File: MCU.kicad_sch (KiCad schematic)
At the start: 17 parts, among them J1 Conn_01x05_Socket, SW1 SW_Push, U1 STM32F405RGT6, Y1 8MHz 10ppm

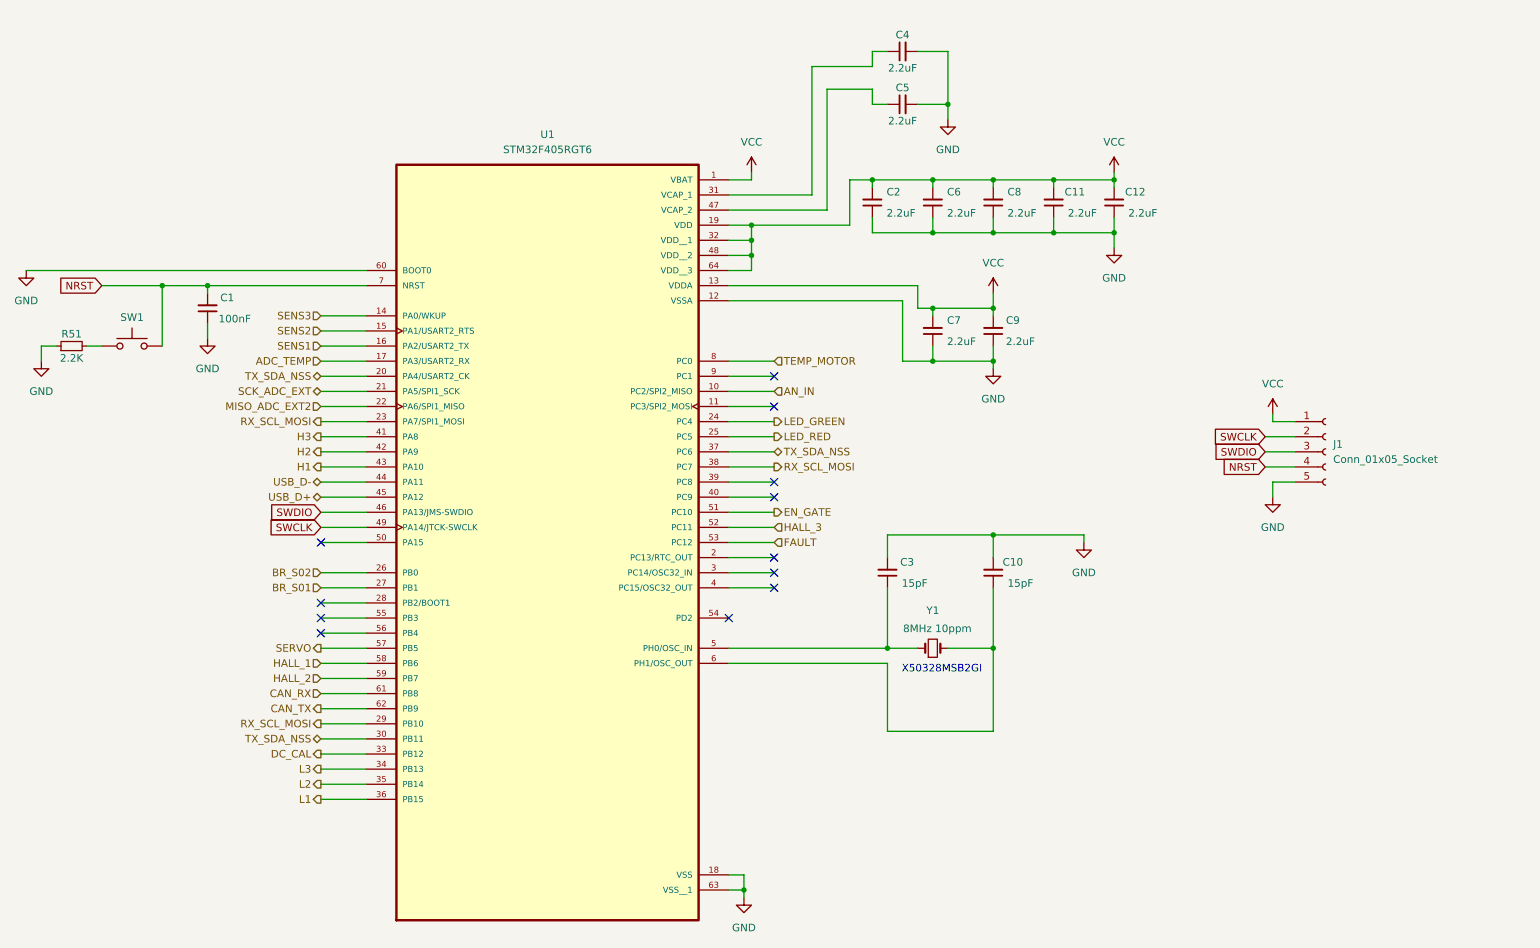
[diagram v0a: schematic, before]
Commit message: finishing+microchecking
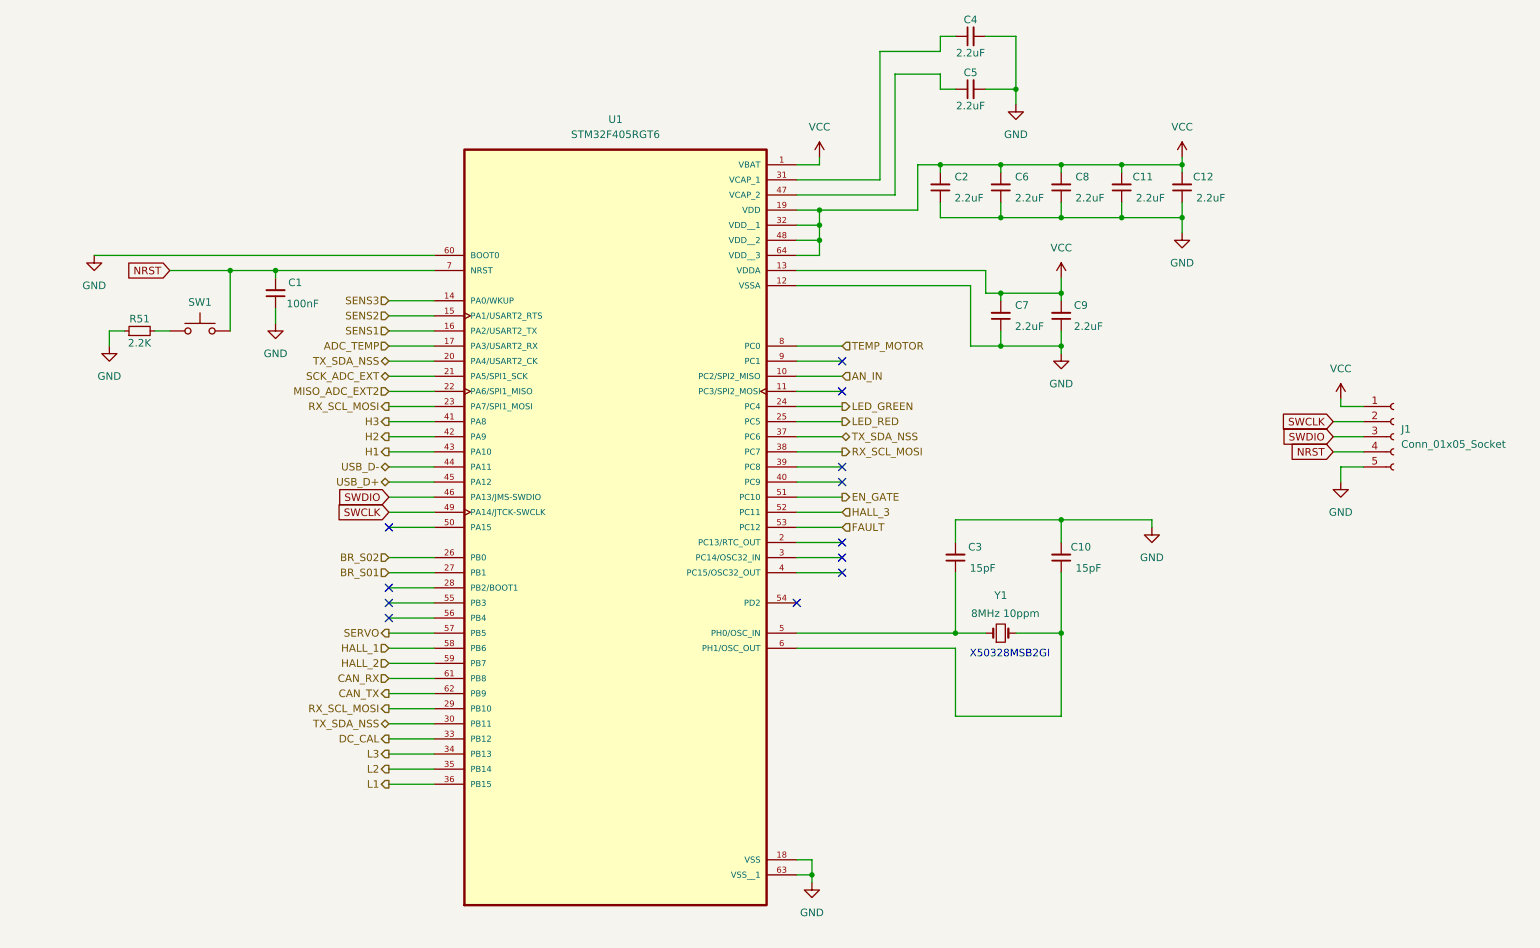
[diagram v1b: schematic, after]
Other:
- moved on the sheet: C1, C10, C11, C12, C2, C3, C4, C5, C6, C7, C8, C9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
